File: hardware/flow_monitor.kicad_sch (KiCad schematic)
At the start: 81 parts, among them J1 Conn_01x04_Pin, J2 USB_C_Receptacle_USB2.0_16P, J3 Conn_01x02_Socket, J4 Conn_01x02_Socket, J5 Conn_01x02_Socket, Q1 2N7002, Q2 IRLML6402, Q3 BC807, Q4 BC817, Q6 2N7002, SW1 1TS005F-2500-5001, SW2 1TS005F-2500-5001, SW3 1TS005F-2500-5001, SW4 1TS005F-2500-5001, SW5 SW_SPDT, U1 USBLC6-2SC6, U2 BQ25185DLHR, U3 CH340C, U4 TPS631000, U5 LMV331, U6 STM32G030C8Tx, U7 EA_DOGS164W-A, Y1 Crystal

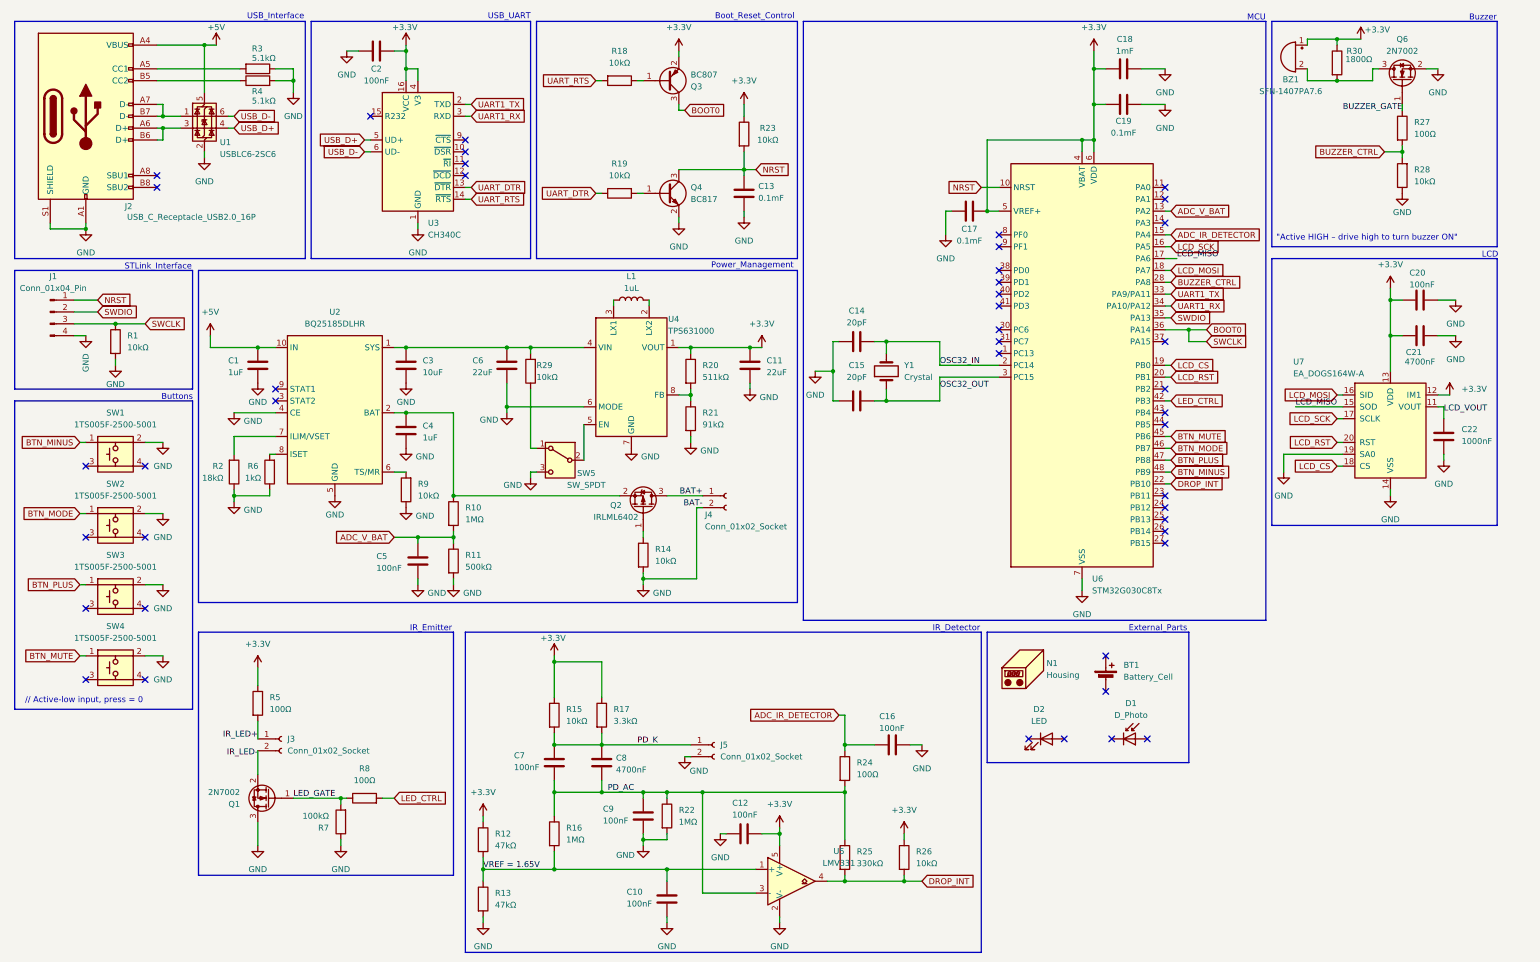
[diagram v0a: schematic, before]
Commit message: small changes
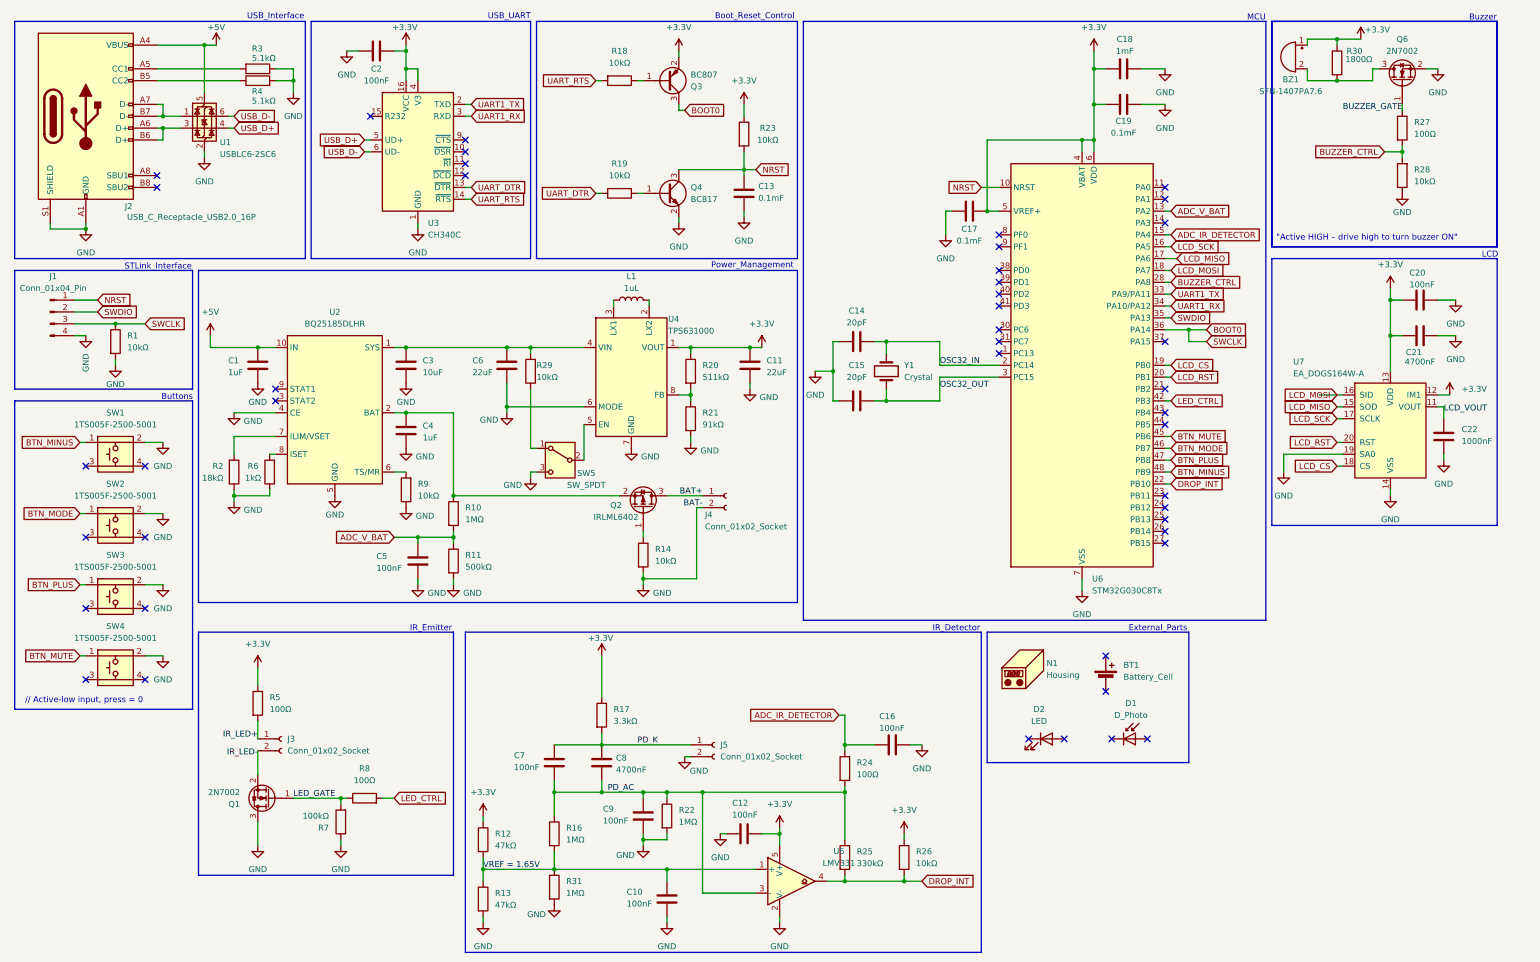
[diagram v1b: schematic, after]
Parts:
- removed R15: 10kΩ, Resistor_SMD:R_0603_1608Metric, symbol Device:R
- added R31: 1MΩ, Resistor_SMD:R_0603_1608Metric, symbol Device:R
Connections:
- net GND: now also R31.2
- net VREF = 1.65V: now also R31.1
